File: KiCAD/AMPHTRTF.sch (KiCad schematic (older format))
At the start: 3 parts

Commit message: Add scfollws.sch
Signed-off-by: John Bradley <flypie@rocketmail.com>
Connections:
- net labels removed: AC
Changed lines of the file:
@@
 $Descr A3 16535 11693
 encoding utf-8
-Sheet 7 32
+Sheet 7 33
 Title "Control Adder Position 6.4"
 Date "2020-10-08"
@@
 Wire Wire Line
 	6075 5050 5725 5050
-$Comp
-L power:AC #PWR0103
-U 1 1 5F304A28
-P 5725 4650
-F 0 "#PWR0103" H 5725 4550 50  0001 C CNN
-F 1 "AC" H 5725 4950 50  0000 C CNN
-F 2 "" H 5725 4650 50  0001 C CNN
-F 3 "" H 5725 4650 50  0001 C CNN
-	1    5725 4650
-	1    0    0    -1
-$EndComp
-$Comp
-L power:AC #PWR0104
-U 1 1 5F3052AC
-P 5725 5050
-F 0 "#PWR0104" H 5725 4950 50  0001 C CNN
-F 1 "AC" H 5725 5350 50  0000 C CNN
-F 2 "" H 5725 5050 50  0001 C CNN
-F 3 "" H 5725 5050 50  0001 C CNN
-	1    5725 5050
-	1    0    0    -1
-$EndComp
 Wire Wire Line
 	6875 4650 7250 4650

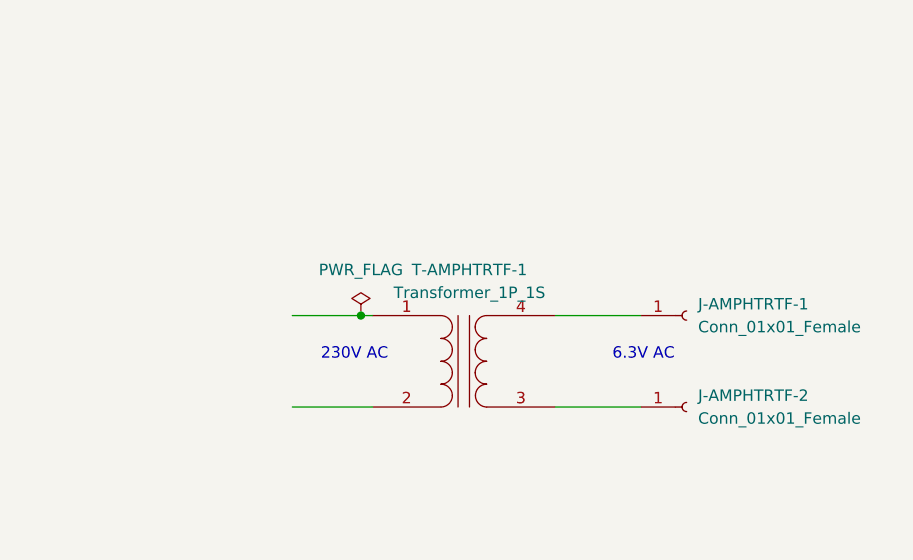
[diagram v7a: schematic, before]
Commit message: Add TYPEWE WRERCCTS YAMP&HVR.
Which com,pletes the first pass. All the pages are done but I haven't checked them yet and there are bound to be errosr.

Signed-off-by: John Bradley <flypie@rocketmail.com>
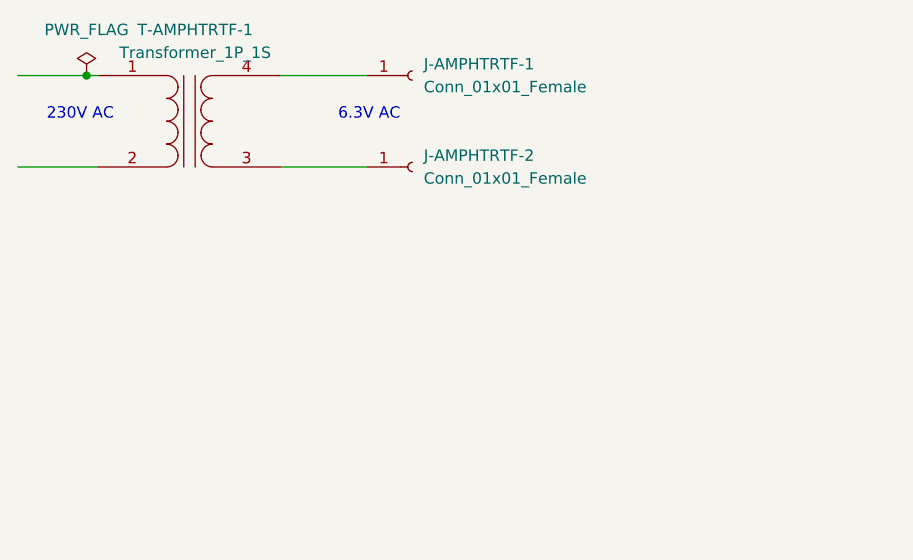
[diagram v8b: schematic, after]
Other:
- moved on the sheet: J-AMPHTRTF-1, J-AMPHTRTF-2, T-AMPHTRTF-1
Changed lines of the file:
@@
 EELAYER 30 0
 EELAYER END
-$Descr A3 16535 11693
+$Descr A4 11693 8268
 encoding utf-8
-Sheet 7 42
+Sheet 7 45
 Title "Control Adder Position 6.4"
 Date "2020-10-08"
@@
 L Device:Transformer_1P_1S T-AMPHTRTF-1
 U 1 1 5F303E4D
-P 6475 4850
-F 0 "T-AMPHTRTF-1" H 6500 5250 50  0000 C CNN
-F 1 "Transformer_1P_1S" H 6500 5150 50  0000 C CNN
-F 2 "SamacSys_Parts_l:FP12950" H 6475 4850 50  0001 C CNN
-F 3 "~" H 6475 4850 50  0001 C CNN
-	1    6475 4850
+P 5275 3800
+F 0 "T-AMPHTRTF-1" H 5300 4200 50  0000 C CNN
+F 1 "Transformer_1P_1S" H 5300 4100 50  0000 C CNN
+F 2 "SamacSys_Parts_l:FP12950" H 5275 3800 50  0001 C CNN
+F 3 "~" H 5275 3800 50  0001 C CNN
+	1    5275 3800
 	1    0    0    -1
 $EndComp
 Wire Wire Line
-	6075 4650 6025 4650
+	4875 3600 4825 3600
 Wire Wire Line
-	6075 5050 5725 5050
+	4875 4000 4525 4000
 Wire Wire Line
-	6875 4650 7250 4650
+	5675 3600 6050 3600
 Wire Wire Line
-	6875 5050 7250 5050
+	5675 4000 6050 4000
 $Comp
 L Connector:Conn_01x01_Female J-AMPHTRTF-1
 U 1 1 5F3065F5
-P 7450 4650
-F 0 "J-AMPHTRTF-1" H 7500 4700 50  0000 L CNN
-F 1 "Conn_01x01_Female" H 7500 4600 50  0000 L CNN
-F 2 "Connector:Banana_Jack_1Pin" H 7450 4650 50  0001 C CNN
-F 3 "~" H 7450 4650 50  0001 C CNN
-	1    7450 4650
+P 6250 3600
+F 0 "J-AMPHTRTF-1" H 6300 3650 50  0000 L CNN
+F 1 "Conn_01x01_Female" H 6300 3550 50  0000 L CNN
+F 2 "Connector:Banana_Jack_1Pin" H 6250 3600 50  0001 C CNN
+F 3 "~" H 6250 3600 50  0001 C CNN
+	1    6250 3600
 	1    0    0    -1
 $EndComp
@@
 L Connector:Conn_01x01_Female J-AMPHTRTF-2
 U 1 1 5F30757C
-P 7450 5050
-F 0 "J-AMPHTRTF-2" H 7500 5100 50  0000 L CNN
-F 1 "Conn_01x01_Female" H 7500 5000 50  0000 L CNN
-F 2 "Connector:Banana_Jack_1Pin" H 7450 5050 50  0001 C CNN
-F 3 "~" H 7450 5050 50  0001 C CNN
-	1    7450 5050
+P 6250 4000
+F 0 "J-AMPHTRTF-2" H 6300 4050 50  0000 L CNN
+F 1 "Conn_01x01_Female" H 6300 3950 50  0000 L CNN
+F 2 "Connector:Banana_Jack_1Pin" H 6250 4000 50  0001 C CNN
+F 3 "~" H 6250 4000 50  0001 C CNN
+	1    6250 4000
 	1    0    0    -1
 $EndComp
@@
 L power:PWR_FLAG #FLG0114
 U 1 1 5F30A8C9
-P 6025 4650
-F 0 "#FLG0114" H 6025 4725 50  0001 C CNN
-F 1 "PWR_FLAG" H 6025 4850 50  0000 C CNN
-F 2 "" H 6025 4650 50  0001 C CNN
-F 3 "~" H 6025 4650 50  0001 C CNN
-	1    6025 4650
+P 4825 3600
+F 0 "#FLG0114" H 4825 3675 50  0001 C CNN
+F 1 "PWR_FLAG" H 4825 3800 50  0000 C CNN
+F 2 "" H 4825 3600 50  0001 C CNN
+F 3 "~" H 4825 3600 50  0001 C CNN
+	1    4825 3600
 	1    0    0    -1
 $EndComp
-Connection ~ 6025 4650
+Connection ~ 4825 3600
 Wire Wire Line
-	6025 4650 5725 4650
-Text Notes 7125 4850 0    50   ~ 0
+	4825 3600 4525 3600
+Text Notes 5925 3800 0    50   ~ 0
 6.3V AC
-Text Notes 5850 4850 0    50   ~ 0
+Text Notes 4650 3800 0    50   ~ 0
 230V AC
 $EndSCHEMATC
